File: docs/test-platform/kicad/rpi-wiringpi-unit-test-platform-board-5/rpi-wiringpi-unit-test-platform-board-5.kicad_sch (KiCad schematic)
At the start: 9 parts, among them J1 JST_IN_PWR, J2 JST_IN_SIG, J3 JST_IN_LCD, J4 JST_OUT_I2C5V, U1 LVLSHIFT_BOB12009

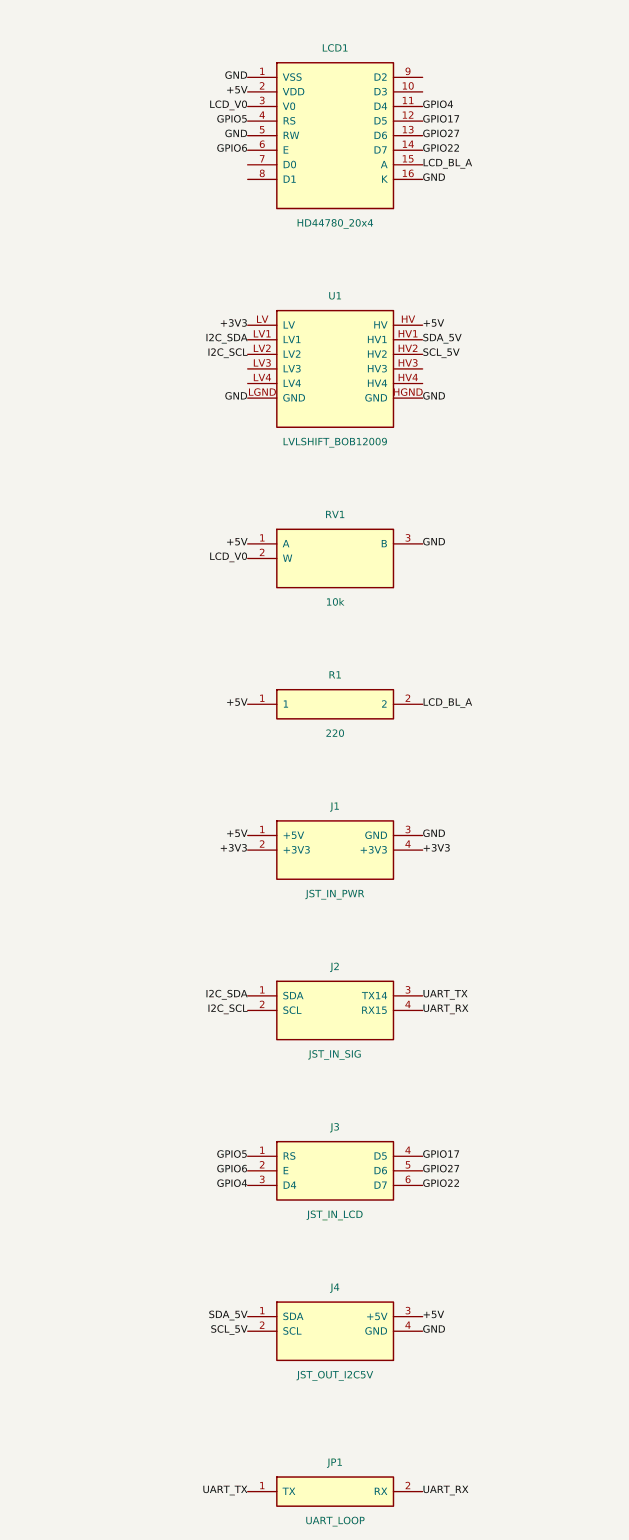
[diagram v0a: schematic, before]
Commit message: Work on test board 5
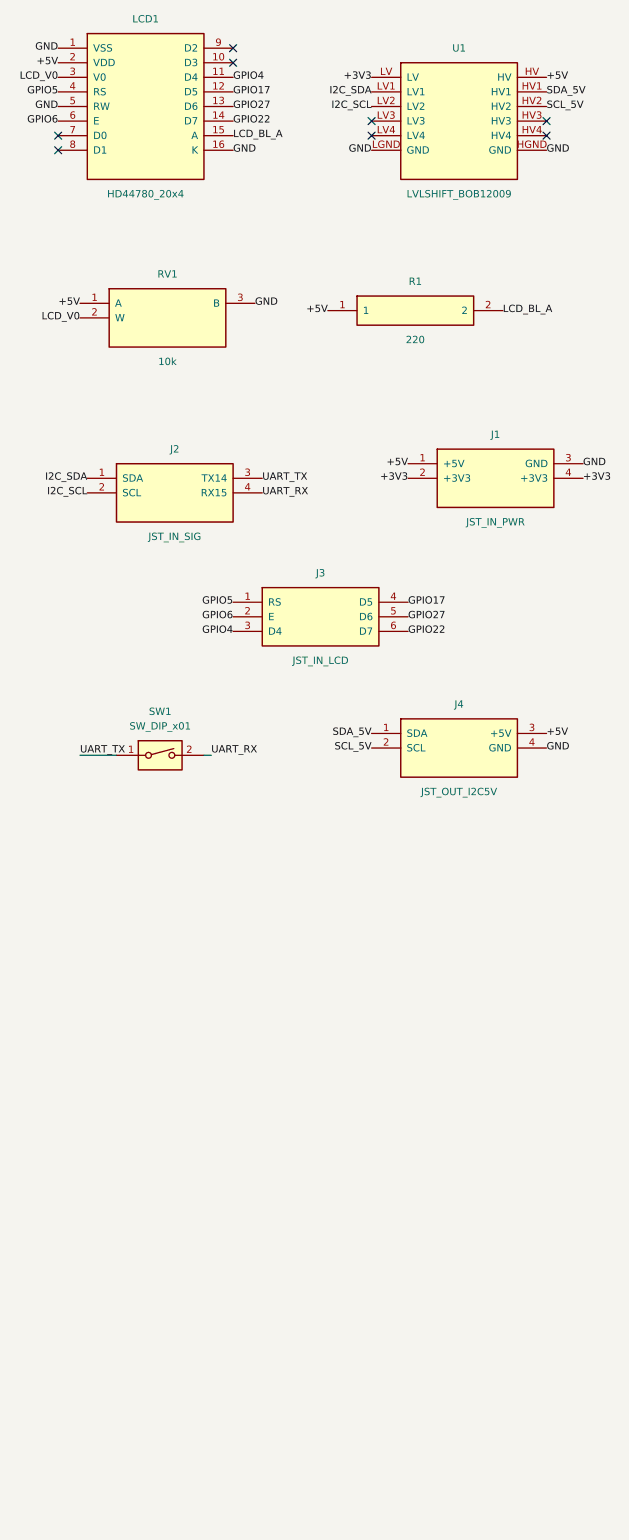
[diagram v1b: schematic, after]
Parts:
- removed JP1: UART_LOOP, rpi-wiringpi-unit-test-platform-board-5:JP1, symbol rpi-wiringpi-unit-test-platform-board-5:JP1
- added SW1: SW_DIP_x01, Button_Switch_THT:SW_DIP_SPSTx01_Slide_9.78x4.72mm_W7.62mm_P2.54mm, symbol Switch:SW_DIP_x01
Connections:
- net UART_RX: now also SW1.2
- net UART_TX: now also SW1.1
- no-connect marks 0 -> 8
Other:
- moved on the sheet: J1, J2, J3, J4, LCD1, R1, RV1, U1
